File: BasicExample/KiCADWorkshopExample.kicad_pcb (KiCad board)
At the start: 2 copper layers, 27.8 x 34.5 mm, 15 parts, among them SW1 TS-1088-AR02016, SW2 TS-1088-AR02016, SW3 TS-1088-AR02016, SW4 TS-1088-AR02016

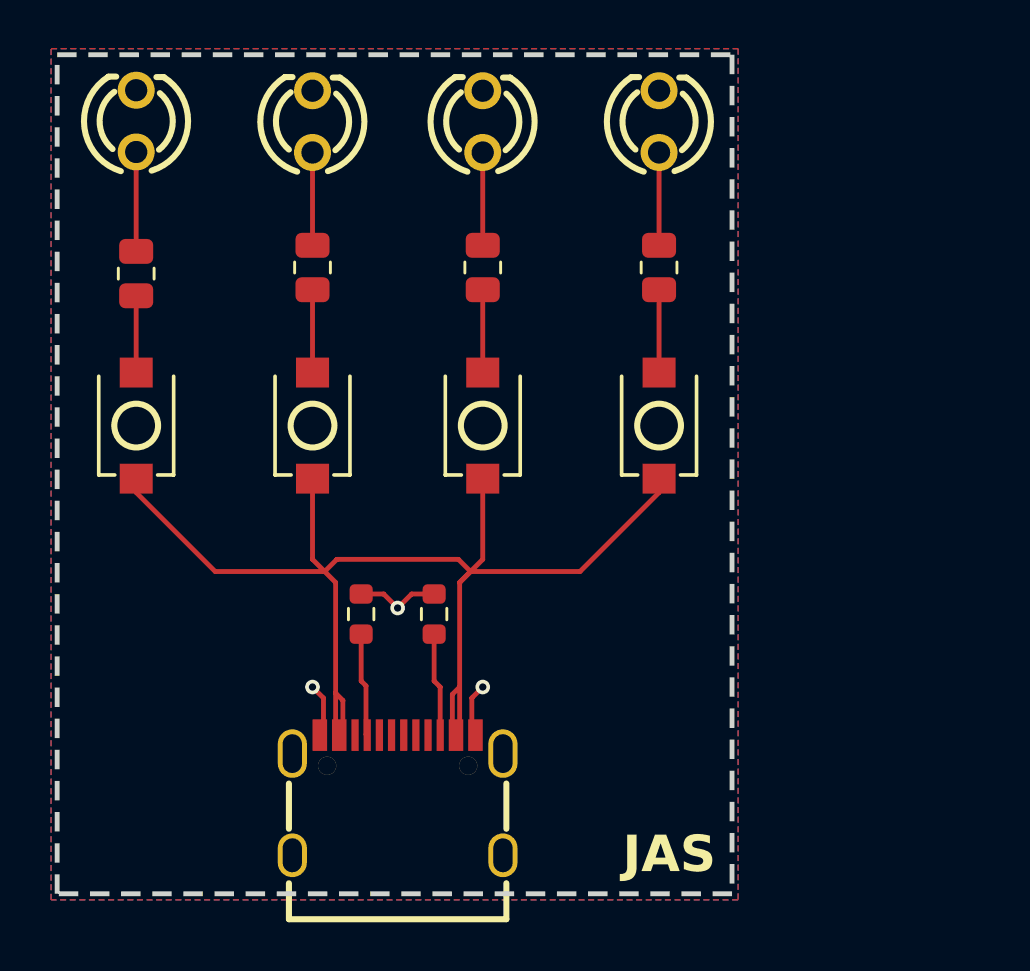
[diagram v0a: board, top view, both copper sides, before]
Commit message: new switch & board in production
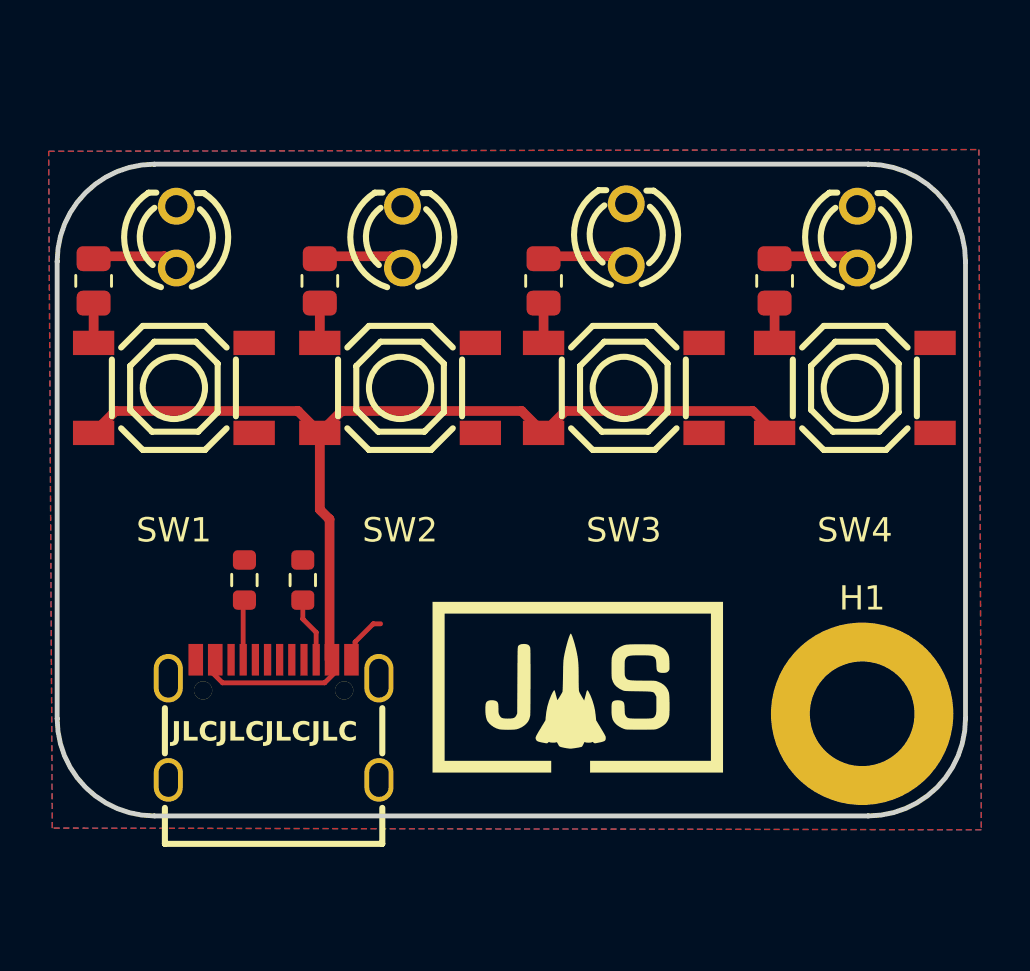
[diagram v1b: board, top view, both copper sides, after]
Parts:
- removed the R5 at (81.8, 124.5)
- added G***: LOGO, Graphics:jas_logo_sm, F.Cu at (99.9, 141.5)
- added H1: MountingHole_Pad, MountingHole:MountingHole_4.3mm_M4_DIN965_Pad, F.Cu at (111.6, 142.6)
- added R2: 120, Resistor_SMD:R_0805_2012Metric, F.Cu at (98.5, 124.8)
- R1, R3, R4: value 250 -> 120
- SW1, SW2, SW3, SW4: value TS-1088-AR02016 -> TS-1187A-B-A-B; footprint ts-1088:SW-SMD_L3.9-W3.0-P4.45 -> ts1088:SW-SMD_4P-L5.1-W5.1-P3.70-LS6.5-TL-2
- moved SW4 29.6 mm to (111.3, 129.2), turned to 180 degrees
- moved SW1 20.0 mm to (83.3, 129.2), turned to 180 degrees
- moved SW3 12.9 mm to (101.8, 129.2), turned to 180 degrees
- moved LED1 9.43 mm to (111.4, 123.0)
- moved R4 9.02 mm to (80.0, 124.8)
- moved LED2 7.51 mm to (101.9, 122.9)
- moved R3 6.72 mm to (89.3, 124.8)
- moved LED3 6.02 mm to (92.7, 123.0)
- moved USBC1 5.97 mm to (87.4, 142.8)
- moved R5 5.58 mm to (88.6, 137.1)
- moved LED4 5.05 mm to (83.4, 123.0)
- moved R6 5.00 mm to (86.2, 137.1)
- moved R1 4.78 mm to (108.0, 124.8)
- moved SW2 3.74 mm to (92.6, 129.2), turned to 180 degrees
- renumbered R6 to R5, R2 to R6
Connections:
- R1 pad 1: Net-(R1-Pad1) -> Net-(SW4-D)
- R3 pad 1: Net-(R3-Pad1) -> Net-(SW2-D)
- R3 pad 2: Net-(LED2-A) -> Net-(LED3-A)
- R4 pad 1: Net-(R4-Pad1) -> Net-(SW1-D)
- R4 pad 2: Net-(LED3-A) -> Net-(LED4-A)
- SW1 pad 1: VBUS -> unconnected-(SW1-A-Pad1)
- SW1 pad 2: Net-(R1-Pad1) -> VBUS
- SW2 pad 1: VBUS -> unconnected-(SW2-A-Pad1)
- SW2 pad 2: Net-(R3-Pad1) -> VBUS
- SW3 pad 1: VBUS -> unconnected-(SW3-A-Pad1)
- SW3 pad 2: Net-(R4-Pad1) -> VBUS
- SW4 pad 1: VBUS -> unconnected-(SW4-A-Pad1)
- SW4 pad 2: Net-(R5-Pad1) -> VBUS
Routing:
- net VBUS: track 52.2 -> 46.2 mm
- net GND: track 7.80 -> 2.09 mm, vias 3 -> 0
- net Net-(R4-Pad1): track 3.41 -> 0.00 mm
- net Net-(R3-Pad1): track 3.41 -> 0.00 mm
- net Net-(R1-Pad1): track 3.41 -> 0.00 mm
- net Net-(R5-Pad1): track 3.16 -> 0.00 mm
- net Net-(USBC1-CC1): track 4.27 -> 2.47 mm
- net Net-(SW4-D): track 0.00 -> 1.74 mm
- net Net-(SW3-D): track 0.00 -> 1.74 mm
- net Net-(SW2-D): track 0.00 -> 1.74 mm
- net Net-(SW1-D): track 0.00 -> 1.74 mm
- net Net-(USBC1-CC2): track 4.26 -> 2.68 mm
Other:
- board size 27.8 x 34.5 mm -> 37.3 x 26.8 mm
- board text added: "JAS KiCAD Workshop Fall 2024"
- board text added: "JLCJLCJLCJLC"
- board text removed: "JAS"
- board text removed: "JAS KiCAD Wrkshp 2024"
